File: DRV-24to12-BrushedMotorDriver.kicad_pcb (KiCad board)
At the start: 2 copper layers, 48 x 38 mm, 34 parts, among them J1 Conn_01x02, J3 Conn_02x04_Odd_Even, U1 DRV8801PWP, U2 TPS5430DDA, U3 ME6211C33M5

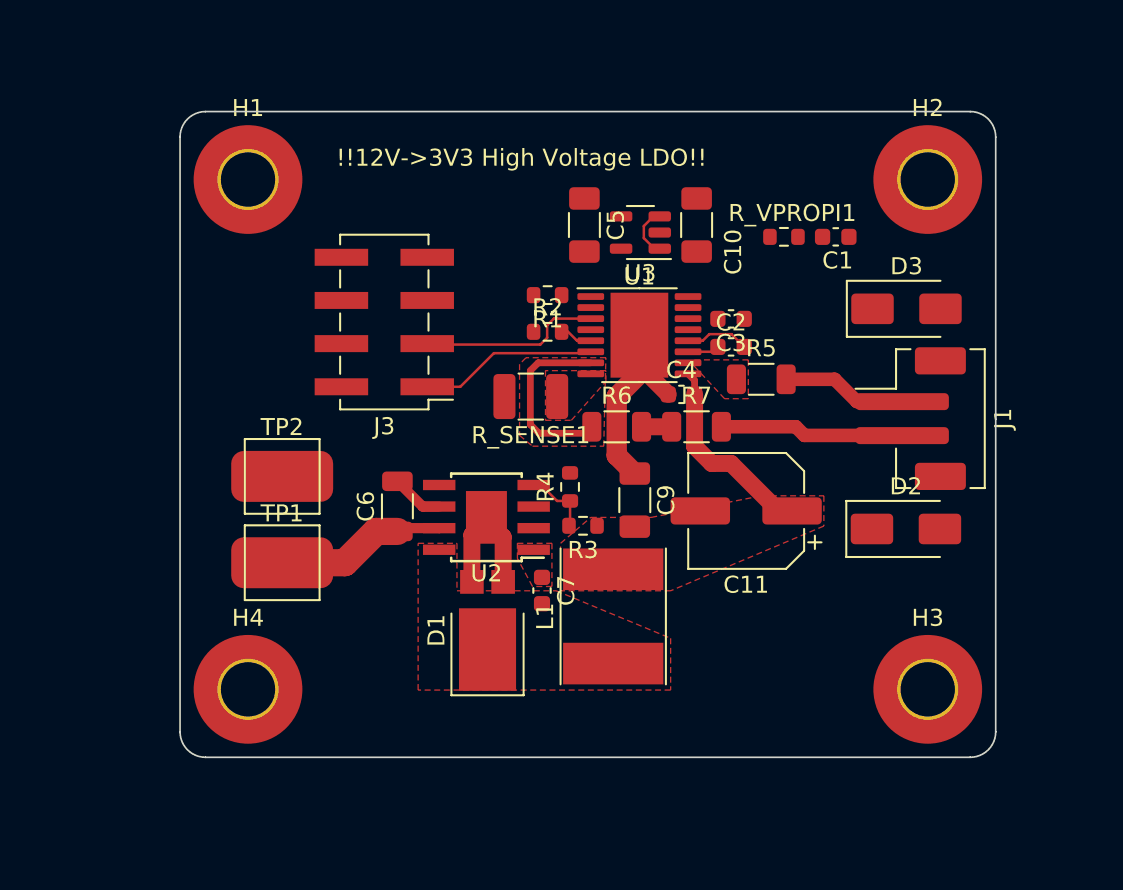
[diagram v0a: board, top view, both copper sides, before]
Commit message: ver1.0 done
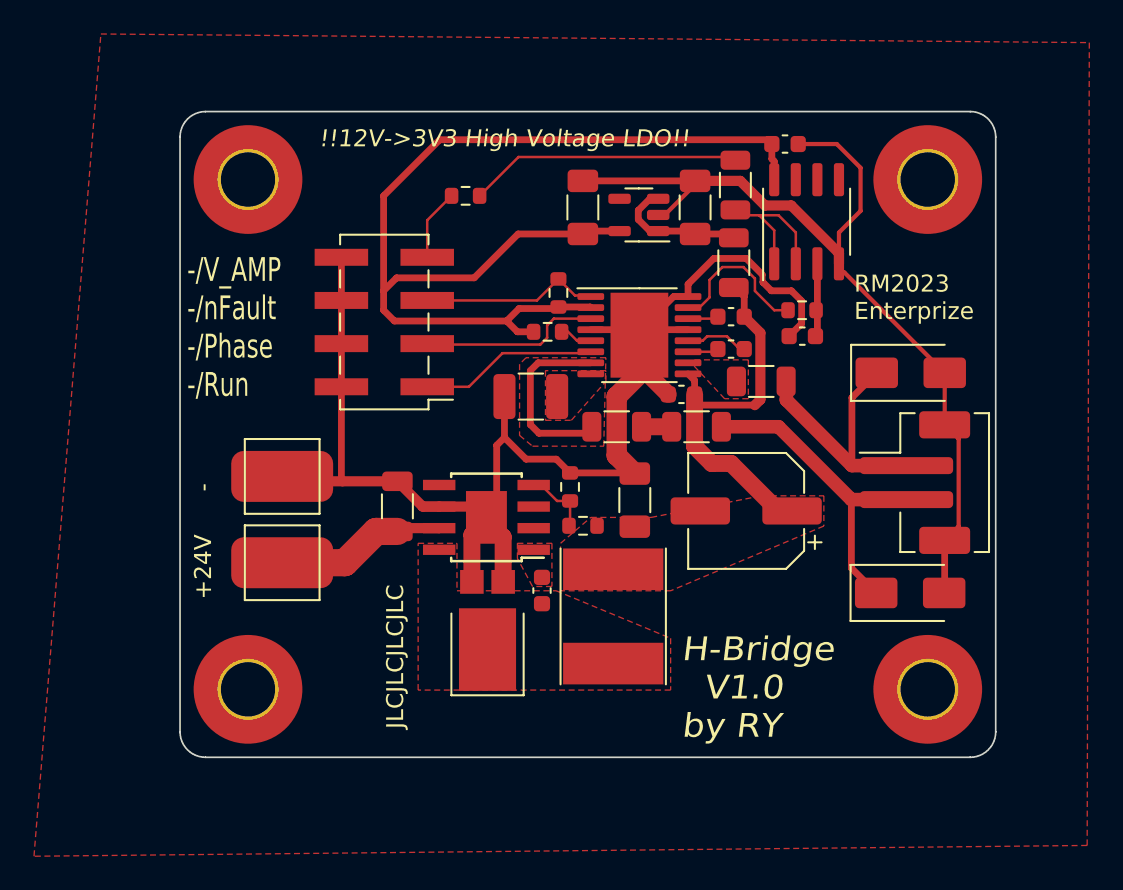
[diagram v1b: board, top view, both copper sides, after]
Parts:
- added C8: 10nF, Capacitor_SMD:C_0603_1608Metric, F.Cu at (236.6, 57.9)
- added R10: 0R 1A, Resistor_SMD:R_1206_3216Metric, F.Cu at (233.6, 64.9)
- added R8: 22R, Resistor_SMD:R_0603_1608Metric, F.Cu at (217.8, 61.0)
- added R9: 0R, Resistor_SMD:R_1206_3216Metric, F.Cu at (233.7, 60.3)
- added U4: LM358, Package_SO:SOIC-8_3.9x4.9mm_P1.27mm, F.Cu at (237.9, 62.5)
- U3: value ME6211C33M5 -> ME6214C33M5G
- moved C1 6.16 mm to (237.6, 69.2), turned to 180 degrees
- moved R_VPROPI1 4.45 mm to (237.6, 67.7)
- moved D2 3.77 mm to (244.0, 84.3)
- moved D3 3.77 mm to (244.0, 71.4)
- moved J1 3.77 mm to (244.2, 77.8)
- moved C5 1.04 mm to (224.7, 61.6)
- moved U3 1.04 mm to (228.0, 62.1)
- moved C10 1.04 mm to (231.3, 61.6)
- moved R1 0.65 mm to (223.3, 66.7), turned to -90 degrees
- moved C2 0.13 mm to (233.4, 70.0)
- moved R5 0.13 mm to (235.2, 71.9)
- moved C3 0.13 mm to (233.4, 68.1)
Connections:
- C10 pad 2: +12V -> Net-(U3-EN)
- J3 pad 7: /VPROPI -> /VPROPI_AMP
- U3 pad 1: +12V -> Net-(U3-EN)
- U3 pad 3: +12V -> Net-(U3-EN)
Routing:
- net GND: track 25.0 -> 139.3 mm
- net +3V3: track 0.00 -> 63.2 mm
- net Net-(R8-Pad1): track 0.00 -> 16.1 mm
- net /NFAULT: track 0.00 -> 10.6 mm
- net Net-(U4A--): track 0.00 -> 9.17 mm
- net +12V: track 14.8 -> 23.6 mm
- net /MOTOR-: track 7.36 -> 16.0 mm
- net Net-(U3-EN): track 0.00 -> 8.47 mm
- net Net-(U1-VPROPI): track 0.00 -> 8.28 mm
- net /MOTOR+: track 10.8 -> 18.7 mm
- net /VPROPI_AMP: track 0.00 -> 4.21 mm
- net /VPROPI: track 0.00 -> 3.80 mm
- net Net-(U1-VCP): track 0.00 -> 1.74 mm
- added copper zone on F.Cu, net GND
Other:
- board text added: "+24V"
- board text added: "-"
- board text added: "-/V_AMP -/nFault -/Phase -/Run"
- board text added: "H-Bridge V1.0 by RY"
- board text added: "JLCJLCJLCJLC"
- board text added: "RM2023 Enterprize"
